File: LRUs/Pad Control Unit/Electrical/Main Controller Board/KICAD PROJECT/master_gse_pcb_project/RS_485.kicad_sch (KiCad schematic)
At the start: 22 parts, among them J8 B3B-XH-A, J9 B3B-XH-A, U17 74LVC1G17, U18 74LVC1G17, U19 SP485EEN-L/TR, U20 SP485EEN-L/TR

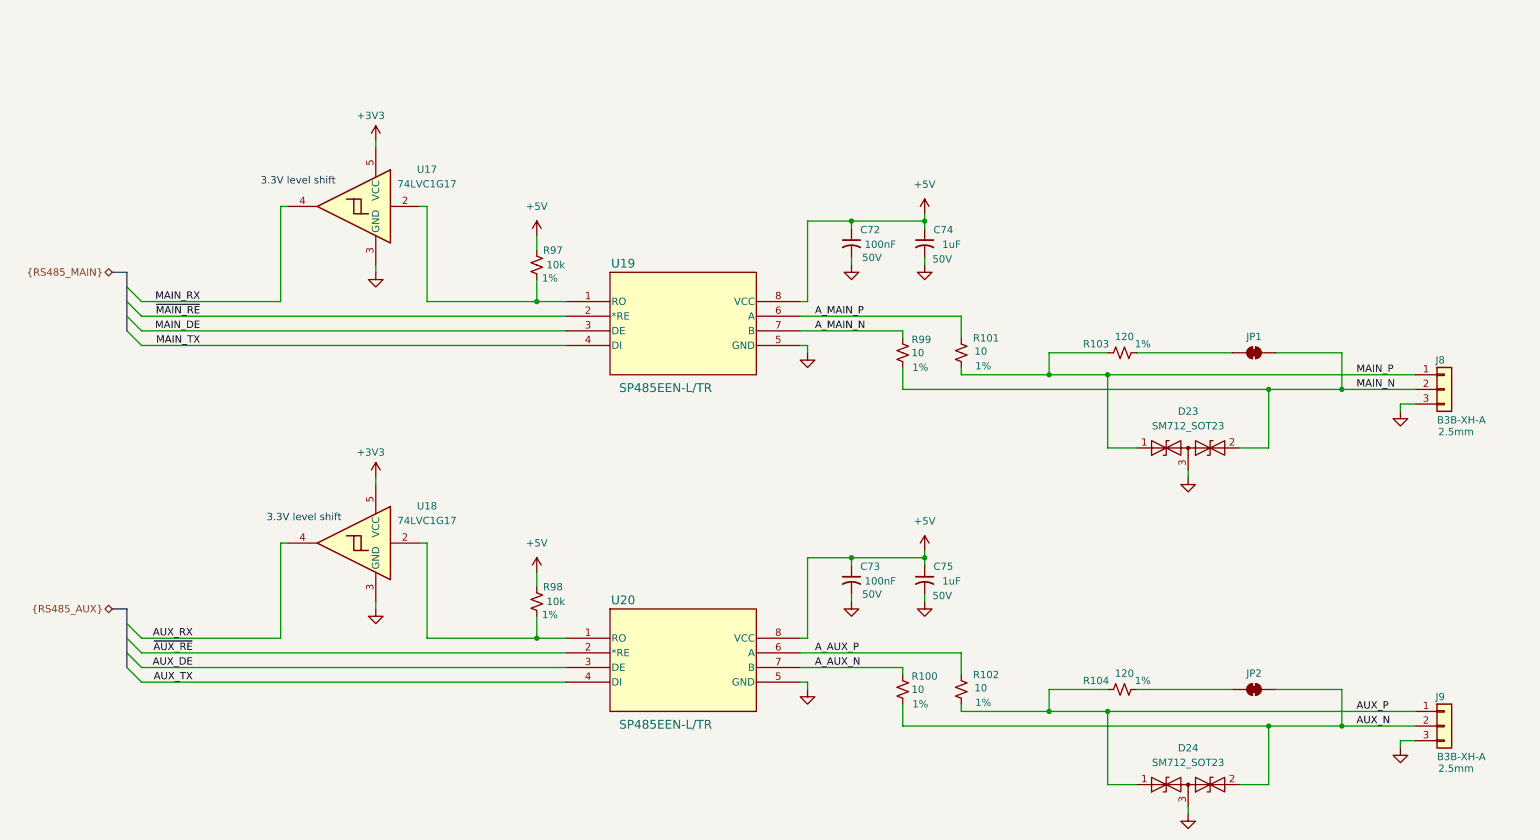
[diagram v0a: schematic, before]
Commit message: Committ latest changes
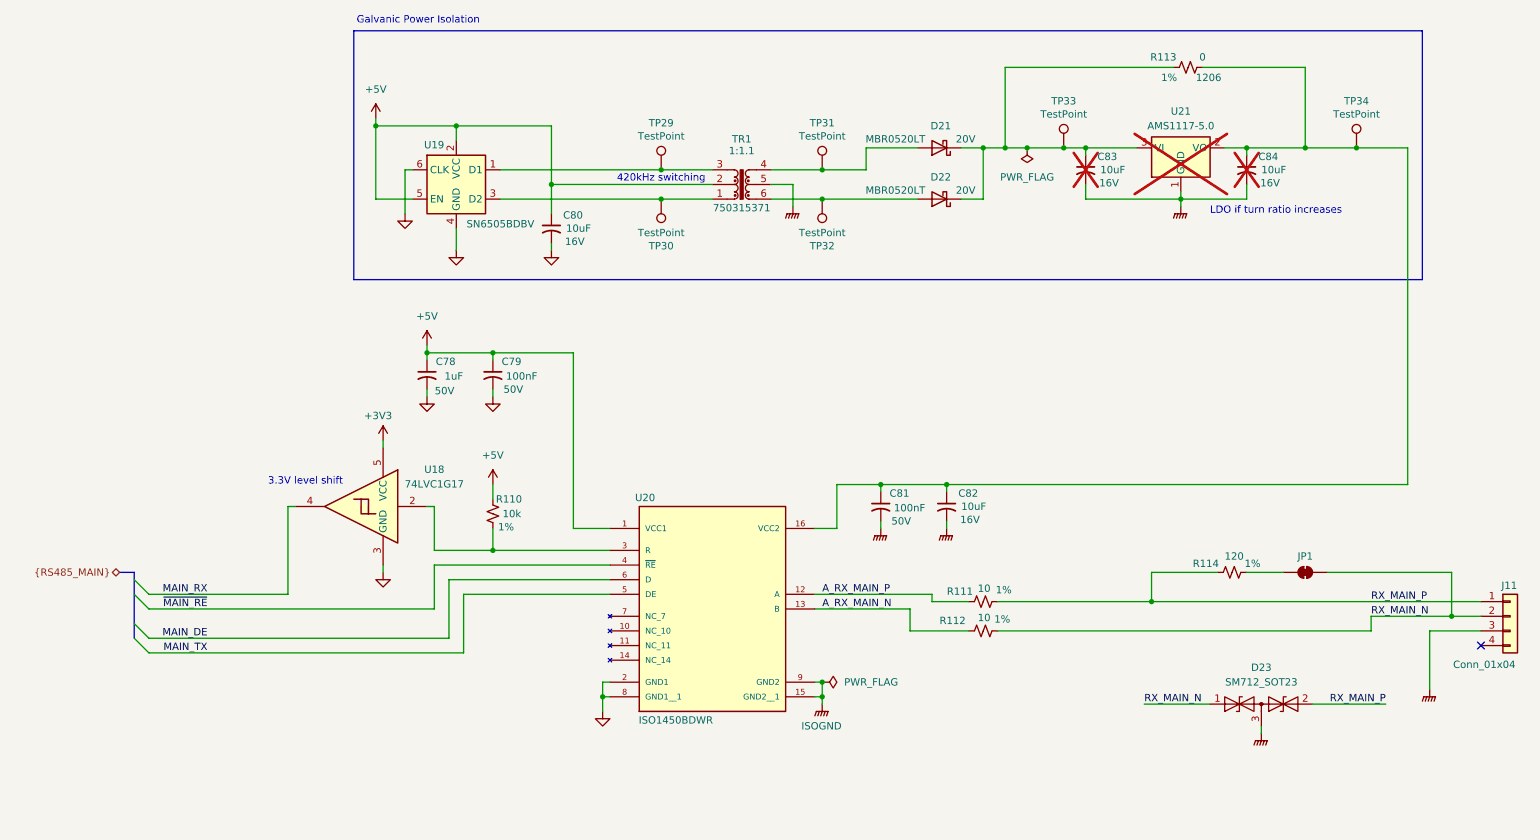
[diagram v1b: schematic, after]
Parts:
- removed C73: 100nF, Capacitor_SMD:C_0402_1005Metric, symbol Device:C_Small_US
- removed C75: 1uF, Capacitor_SMD:C_0805_2012Metric, symbol Device:C_Small_US
- removed D24: SM712_SOT23, Package_TO_SOT_SMD:SOT-23, symbol Diode:SM712_SOT23
- removed J8, J9: B3B-XH-A, Connector_JST:JST_XH_B3B-XH-A_1x03_P2.50mm_Vertical, symbol Connector_Generic:Conn_01x03
- removed JP2: SolderJumper_2_Bridged, Jumper:SolderJumper-2_P1.3mm_Bridged_RoundedPad1.0x1.5mm, symbol Jumper:SolderJumper_2_Bridged
- removed R100, R102: 10, Resistor_SMD:R_0402_1005Metric, symbol Device:R_Small_US
- removed R104: 120, Resistor_SMD:R_0402_1005Metric, symbol Device:R_Small_US
- removed R98: 10k, Resistor_SMD:R_0603_1608Metric, symbol Device:R_Small_US
- removed U18: 74LVC1G17, Package_TO_SOT_SMD:SOT-23-5_HandSoldering, symbol 74xGxx:74LVC1G17
- removed U19, U20: SP485EEN-L/TR, footprints:NSOIC-8, symbol symbols:SP485EEN-L_TR
- added C80, C82, C83, C84: 10uF, Capacitor_SMD:C_0805_2012Metric, symbol Device:C_Small_US
- added C81: 100nF, Capacitor_SMD:C_0402_1005Metric, symbol Device:C_Small_US
- added D21, D22: MBR0520LT, Diode_SMD:D_SOD-123, symbol Diode:MBR0520LT
- added J11: Conn_01x04, Connector_Molex:Molex_Micro-Fit_3.0_43650-0415_1x04_P3.00mm_Vertical, symbol Connector_Generic:Conn_01x04
- added R113: 0, Resistor_SMD:R_1206_3216Metric, symbol Device:R_Small_US
- added TP29, TP30, TP31, TP32, TP33, TP34: TestPoint, TestPoint:TestPoint_Pad_D2.0mm, symbol Connector:TestPoint
- added TR1: 750315371, Transformer_SMD:Transformer_Wuerth_750315371, symbol Transformer:Wuerth_750315371
- added U19: SN6505BDBV, Package_TO_SOT_SMD:SOT-23-6, symbol Power_Management:SN6505BDBV
- added U20: ISO1450BDWR, footprints:SOIC127P1030X265-16N, symbol symbols:ISO1450BDWR
- added U21: AMS1117-5.0, Package_TO_SOT_SMD:SOT-223-3_TabPin2, symbol Regulator_Linear:AMS1117-5.0
- renumbered C74 to C78, C72 to C79, R97 to R110, R101 to R111, R99 to R112, R103 to R114, U17 to U18
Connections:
- net +5V: now also C80.1, TR1.2, U19.2 (VCC), U19.5 (EN), U20.1 (VCC1)
- net GND: now also C80.2, U19.4 (GND), U19.6 (CLK), U20.2 (GND1), U20.8 (GND1__1); no longer D23.3 (common)
- net MAIN_DE: now also U20.6 (D)
- net MAIN_TX: now also U20.5 (DE)
- net ~{MAIN_RE}: now also U20.4 (~{RE})
- net at R110.2, U18.2: now also U20.3 (R)
- net A_MAIN_N renamed A_RX_MAIN_N
- net A_RX_MAIN_N: now also U20.13 (B)
- net A_MAIN_P renamed A_RX_MAIN_P
- net A_RX_MAIN_P: now also U20.12 (A)
- net MAIN_N renamed RX_MAIN_N
- net RX_MAIN_N: now also D23.1 (A1), J11.2 (Pin_2); no longer D23.2 (A2)
- net MAIN_P renamed RX_MAIN_P
- net RX_MAIN_P: now also D23.2 (A2), J11.1 (Pin_1); no longer D23.1 (A1)
- new net: TP30.1, TR1.1, U19.3 (D2)
- new net: TP29.1, TR1.3, U19.1 (D1)
- new net: C83.1, D21.1 (K), D22.1 (K), R113.2, TP33.1, U21.3 (VI)
- new net: D21.2 (A), TP31.1, TR1.4
- new net: C81.1, C82.1, C84.1, R113.1, TP34.1, U20.16 (VCC2), U21.2 (VO)
- new net: D22.2 (A), TP32.1, TR1.6
- new net ISOGND: C81.2, C82.2, C83.2, C84.2, D23.3 (common), J11.3 (Pin_3), TR1.5, U20.15 (GND2__1), U20.9 (GND2), U21.1 (GND)
- no-connect marks 0 -> 1
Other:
- note added: "420kHz switching"
- note added: "Galvanic Power Isolation"
- note added: "LDO if turn ratio increases"
- moved on the sheet: C78, C79, D23, JP1, R110, R111, R112, R114, U18
